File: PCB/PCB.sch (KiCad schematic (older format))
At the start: 20 parts, among them J1 AVR-ISP-6, SW1 SW_Push

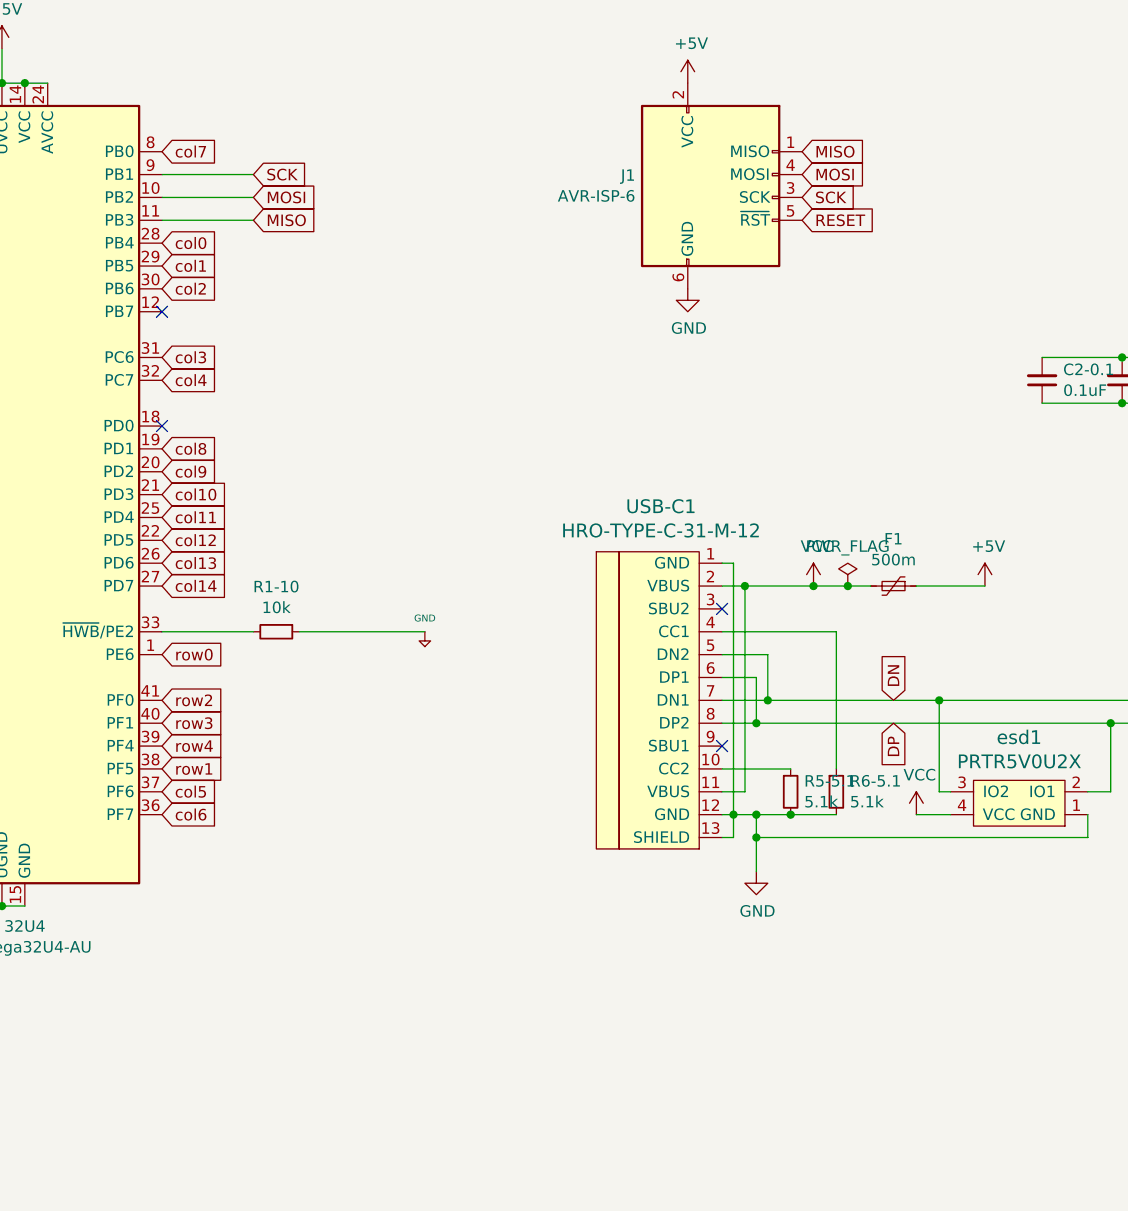
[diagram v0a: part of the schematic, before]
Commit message: PCB Done
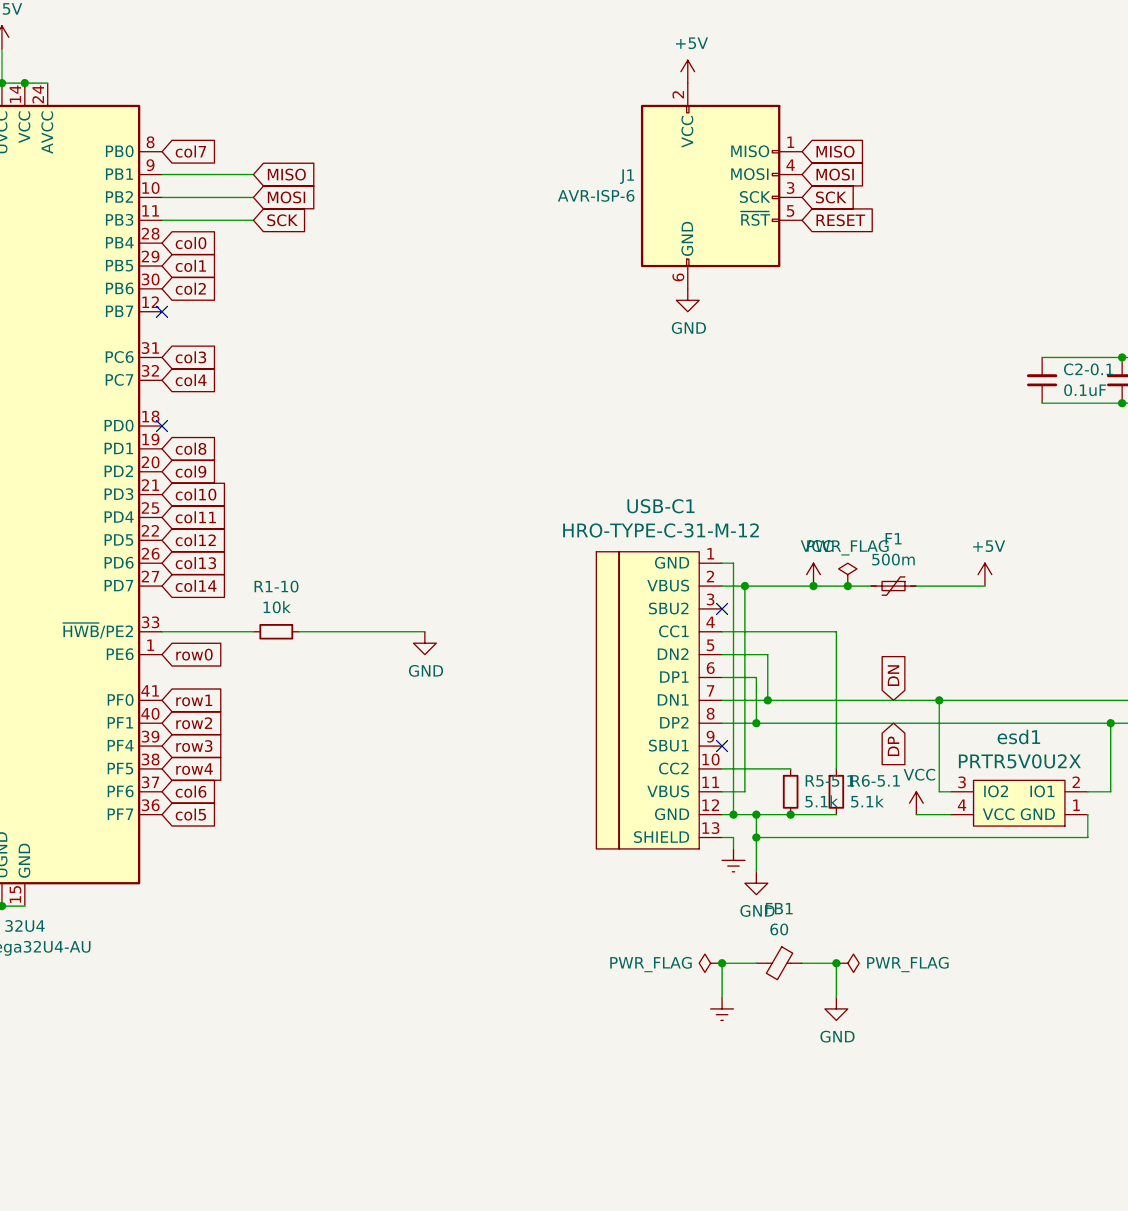
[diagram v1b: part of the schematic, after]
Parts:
- added FB1: 60, Inductor_SMD:L_0805_2012Metric_Pad1.05x1.20mm_HandSolder, symbol Device:Ferrite_Bead_Small
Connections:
- net +5V: no longer R1-10.1
- net GND: now also R1-10.1, FB1.1; no longer USB-C1.13 (SHIELD)
- net MISO: now also 32U4.9 (PB1); no longer 32U4.11 (PB3)
- net SCK: now also 32U4.11 (PB3); no longer 32U4.9 (PB1)
- net col5: now also 32U4.36 (PF7); no longer 32U4.37 (PF6)
- net col6: now also 32U4.37 (PF6); no longer 32U4.36 (PF7)
- net row1: now also 32U4.41 (PF0); no longer 32U4.38 (PF5)
- net row2: now also 32U4.40 (PF1); no longer 32U4.41 (PF0)
- net row3: now also 32U4.39 (PF4); no longer 32U4.40 (PF1)
- net row4: now also 32U4.38 (PF5); no longer 32U4.39 (PF4)
- new net Earth: FB1.2, USB-C1.13 (SHIELD)
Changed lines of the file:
@@
 	0    1    1    0
-$EndComp
-$Comp
-L keyboard_parts:GND #PWR0103
-U 1 1 61E9EDC0
-P 5250 4250
-F 0 "#PWR0103" H 5250 4300 20  0001 C CNN
-F 1 "GND" H 5250 4309 30  0000 C CNN
-F 2 "" H 5250 4250 60  0000 C CNN
-F 3 "" H 5250 4250 60  0000 C CNN
-	1    5250 4250
-	1    0    0    -1
 $EndComp
 Wire Wire Line
@@
 Text GLabel 6900 2450 2    50   Input ~ 0
 RESET
-Text GLabel 4500 2250 2    50   Input ~ 0
+Text GLabel 4500 2450 2    50   Input ~ 0
 SCK
 Text GLabel 4500 2350 2    50   Input ~ 0
 MOSI
-Text GLabel 4500 2450 2    50   Input ~ 0
+Text GLabel 4500 2250 2    50   Input ~ 0
 MISO
 $Comp
@@
 	6550 5050 6600 5050
 Connection ~ 6600 5050
-Wire Wire Line
-	6600 5050 6600 5150
 $Comp
 L power:VCC #PWR0113
@@
 Text GLabel 4100 4350 2    50   Input ~ 0
 row0
+Text GLabel 4100 4650 2    50   Input ~ 0
+row2
+Text GLabel 4100 4750 2    50   Input ~ 0
+row3
+Text GLabel 4100 4850 2    50   Input ~ 0
+row4
 Text GLabel 4100 4550 2    50   Input ~ 0
-row2
-Text GLabel 4100 4650 2    50   Input ~ 0
-row3
-Text GLabel 4100 4750 2    50   Input ~ 0
-row4
-Text GLabel 4100 4850 2    50   Input ~ 0
 row1
+Text GLabel 4100 5050 2    50   Input ~ 0
+col5
 Text GLabel 4100 4950 2    50   Input ~ 0
-col5
-Text GLabel 4100 5050 2    50   Input ~ 0
 col6
 Text GLabel 2850 2150 3    50   Input ~ 0
@@
 $EndComp
 $Comp
-L power:GND #PWR0111
-U 1 1 6247EF75
-P 6700 5300
-F 0 "#PWR0111" H 6700 5050 50  0001 C CNN
-F 1 "GND" H 6705 5127 50  0000 C CNN
-F 2 "" H 6700 5300 50  0001 C CNN
-F 3 "" H 6700 5300 50  0001 C CNN
-	1    6700 5300
-	1    0    0    -1
-$EndComp
-$Comp
 L power:GND #PWR0115
 U 1 1 6247FB74
@@
 Text GLabel 7300 4650 3    50   Input ~ 0
 DP
+$Comp
+L power:GND #PWR0103
+U 1 1 624F6E3A
+P 5250 4250
+F 0 "#PWR0103" H 5250 4000 50  0001 C CNN
+F 1 "GND" H 5255 4077 50  0000 C CNN
+F 2 "" H 5250 4250 50  0001 C CNN
+F 3 "" H 5250 4250 50  0001 C CNN
+	1    5250 4250
+	1    0    0    -1
+$EndComp
+$Comp
+L power:Earth #PWR0111
+U 1 1 6259718E
+P 6600 5200
+F 0 "#PWR0111" H 6600 4950 50  0001 C CNN
+F 1 "Earth" H 6600 5050 50  0001 C CNN
+F 2 "" H 6600 5200 50  0001 C CNN
+F 3 "~" H 6600 5200 50  0001 C CNN
+	1    6600 5200
+	1    0    0    -1
+$EndComp
+$Comp
+L Device:Ferrite_Bead_Small FB1
+U 1 1 62599F62
+P 6800 5700
+F 0 "FB1" V 6563 5700 50  0000 C CNN
+F 1 "60" V 6654 5700 50  0000 C CNN
+F 2 "Inductor_SMD:L_0805_2012Metric_Pad1.05x1.20mm_HandSolder" V 6730 5700 50  0001 C CNN
+F 3 "~" H 6800 5700 50  0001 C CNN
+	1    6800 5700
+	0    1    1    0
+$EndComp
+$Comp
+L power:PWR_FLAG #FLG0101
+U 1 1 6259B007
+P 6550 5700
+F 0 "#FLG0101" H 6550 5775 50  0001 C CNN
+F 1 "PWR_FLAG" V 6550 5827 50  0000 L CNN
+F 2 "" H 6550 5700 50  0001 C CNN
+F 3 "~" H 6550 5700 50  0001 C CNN
+	1    6550 5700
+	0    -1   -1   0
+$EndComp
+$Comp
+L power:PWR_FLAG #FLG0104
+U 1 1 6259BA2D
+P 7050 5700
+F 0 "#FLG0104" H 7050 5775 50  0001 C CNN
+F 1 "PWR_FLAG" V 7050 5828 50  0000 L CNN
+F 2 "" H 7050 5700 50  0001 C CNN
+F 3 "~" H 7050 5700 50  0001 C CNN
+	1    7050 5700
+	0    1    1    0
+$EndComp
+Wire Wire Line
+	6550 5700 6700 5700
+Wire Wire Line
+	6900 5700 7050 5700
+$Comp
+L power:Earth #PWR0117
+U 1 1 625A1153
+P 6550 5850
+F 0 "#PWR0117" H 6550 5600 50  0001 C CNN
+F 1 "Earth" H 6550 5700 50  0001 C CNN
+F 2 "" H 6550 5850 50  0001 C CNN
+F 3 "~" H 6550 5850 50  0001 C CNN
+	1    6550 5850
+	1    0    0    -1
+$EndComp
+Wire Wire Line
+	6550 5850 6550 5700
+Connection ~ 6550 5700
+$Comp
+L power:GND #PWR0118
+U 1 1 625A4186
+P 7050 5850
+F 0 "#PWR0118" H 7050 5600 50  0001 C CNN
+F 1 "GND" H 7055 5677 50  0000 C CNN
+F 2 "" H 7050 5850 50  0001 C CNN
+F 3 "" H 7050 5850 50  0001 C CNN
+	1    7050 5850
+	1    0    0    -1
+$EndComp
+Wire Wire Line
+	7050 5700 7050 5850
+Connection ~ 7050 5700
+Wire Wire Line
+	6600 5150 6600 5200
+$Comp
+L power:GND #PWR?
+U 1 1 625AE0FC
+P 6700 5300
+F 0 "#PWR?" H 6700 5050 50  0001 C CNN
+F 1 "GND" H 6705 5127 50  0000 C CNN
+F 2 "" H 6700 5300 50  0001 C CNN
+F 3 "" H 6700 5300 50  0001 C CNN
+	1    6700 5300
+	1    0    0    -1
+$EndComp
 $EndSCHEMATC
